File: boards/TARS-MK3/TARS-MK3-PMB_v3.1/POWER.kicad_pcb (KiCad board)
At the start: 2 copper layers, 86 x 79.1 mm, 57 parts, among them J1 Conn_02x12_Odd_Even, J2 Conn_02x12_Odd_Even, J3 Conn_02x12_Odd_Even, J4 Conn_02x12_Odd_Even, J5 AVRISP, U1 LK112M33TR, U2 ATmega328P-A, U3 D36V50F6, U4 D36V50F6, U5 D36V28F9, U6 D36V28F3, U7 D24V50F5, Y1 8Mhz

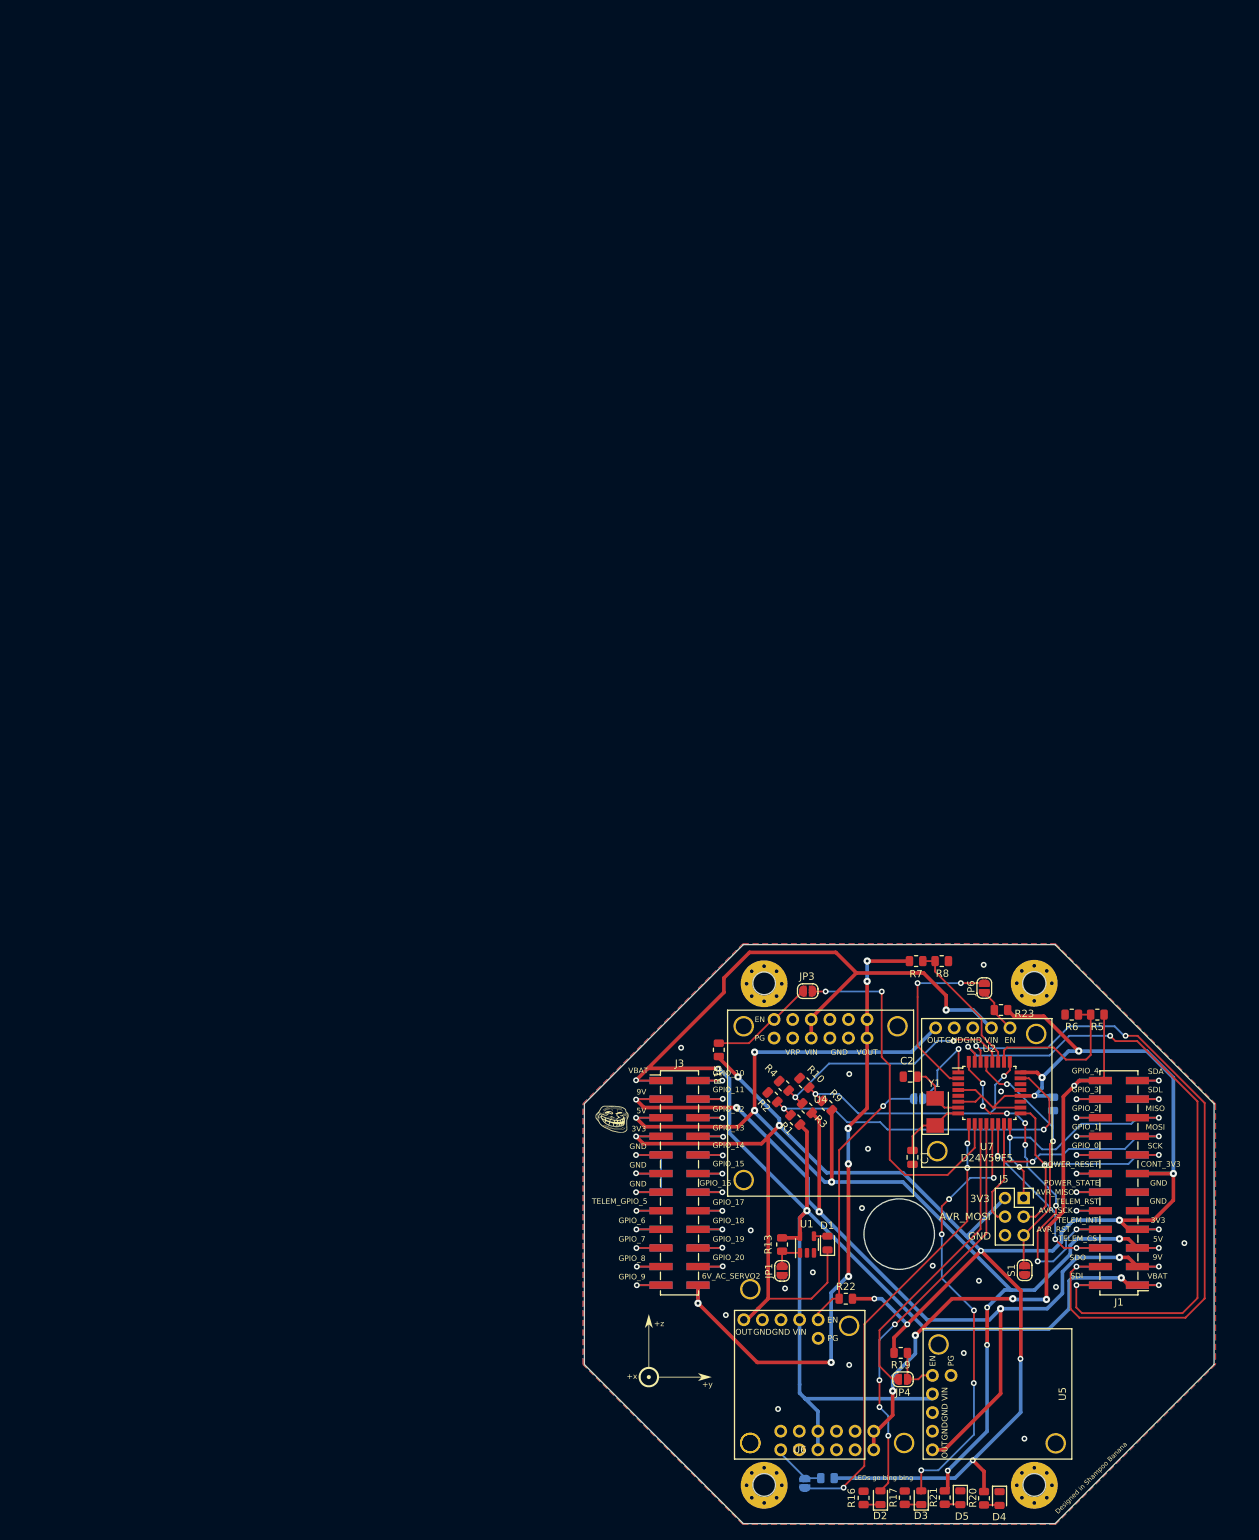
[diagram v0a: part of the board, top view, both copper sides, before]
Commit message: finished template stuff
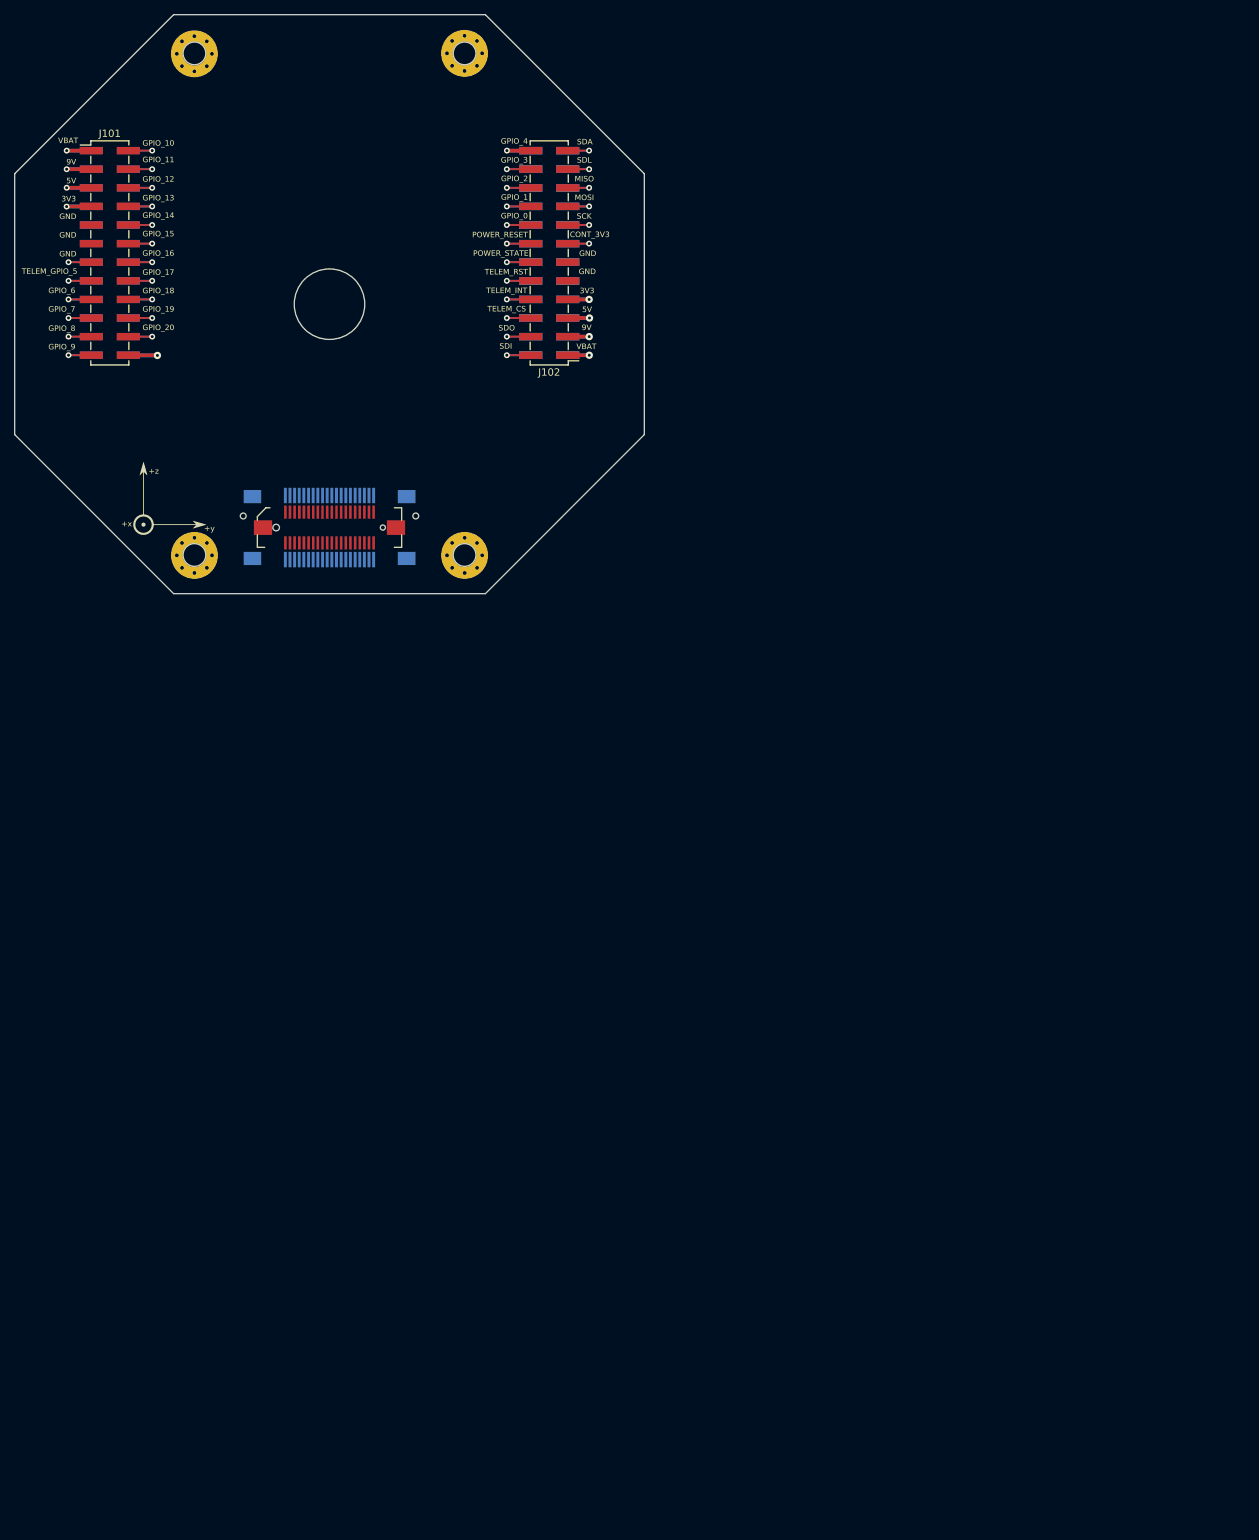
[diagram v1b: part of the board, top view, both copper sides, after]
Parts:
- removed C1, C2: LOAD_C, Capacitor_SMD:C_0805_2012Metric
- removed D1: D, Diode_SMD:D_0805_2012Metric
- removed D2: GREEN, LED_SMD:LED_0805_2012Metric
- removed D3: ORANGE, LED_SMD:LED_0805_2012Metric
- removed D4: LED, LED_SMD:LED_0805_2012Metric
- removed D5: LED, Diode_SMD:D_0805_2012Metric
- removed the G*** at (38.6, 111.3)
- removed the G*** at (101.9, 95.2)
- removed the G*** at (105.1, 141.3)
- removed the G*** at (95.1, 152.1)
- removed J1, J2, J3, J4: Conn_02x12_Odd_Even, Connector_PinHeader_2.54mm:PinHeader_2x12_P2.54mm_Vertical_SMD
- removed J5: AVRISP, Connector_PinSocket_2.54mm:PinSocket_2x03_P2.54mm_Vertical
- removed JP1, JP2, JP3, JP4, JP5, JP6: Jumper_2_Open, Jumper:SolderJumper-2_P1.3mm_Open_RoundedPad1.0x1.5mm
- removed R1, R3: 200kOhm, Resistor_SMD:R_0805_2012Metric
- removed R10, R13, R14, R15, R19, R2, R22, R23, R4, R5, R6, R7, R8, R9: 100kOhm, Resistor_SMD:R_0805_2012Metric
- removed R16, R17: 150Ω, Resistor_SMD:R_0805_2012Metric
- removed R18: 10k, Resistor_SMD:R_0805_2012Metric
- removed R20, R21: 1k, Resistor_SMD:R_0805_2012Metric
- removed the REF** at (96.2, 92.7)
- removed the REF** at (59.3, 92.8)
- removed the REF** at (59.4, 161.3)
- removed the REF** at (96.2, 161.3)
- removed S1: Reset, Jumper:SolderJumper-2_P1.3mm_Open_RoundedPad1.0x1.5mm
- removed U1: LK112M33TR, Package_TO_SOT_SMD:SOT-23-5
- removed U2: ATmega328P-A, Package_QFP:TQFP-32_7x7mm_P0.8mm
- removed U3, U4: D36V50F6, D36V50F6:D36V50F6-TARS
- removed U5: D36V28F9, D36V28F3:D36V28F3
- removed U6: D36V28F3, D36V28F3:D36V28F3
- removed U7: D24V50F5, D24V50F5:D24V50F5
- removed Y1: 8Mhz, Crystal:Crystal_SMD_5032-2Pin_5.0x3.2mm
- added J101: Conn_02x12_Odd_Even, Connector_PinHeader_2.54mm:PinHeader_2x12_P2.54mm_Vertical_SMD, F.Cu at (-30.0, -7.00)
- added J102: Conn_02x12_Odd_Even, Connector_PinHeader_2.54mm:PinHeader_2x12_P2.54mm_Vertical_SMD, F.Cu at (30.0, -7.00)
- added J102, J104: Conn_02x12_Odd_Even, Connector_PinHeader_2.54mm:PinHeader_2x12_P2.54mm_Vertical_SMD, B.Cu at (30.0, -7.00)
- added J103: Conn_02x12_Odd_Even, Connector_PinHeader_2.54mm:PinHeader_2x12_P2.54mm_Vertical_SMD, B.Cu at (-30.0, -7.00)
- added J105: Receptacle, Connector_ISS:2091680401, B.Cu at (0.00, 30.5)
- added J106: 536270474, Connector_ISS:536270474, F.Cu at (0.00, 30.5)
- added REF**: MountingHole_3.2mm_M3_Pad_Via, MountingHole:MountingHole_3.2mm_M3_Pad_Via, F.Cu at (-18.4, 34.3)
- added REF**: MountingHole_3.2mm_M3_Pad_Via, MountingHole:MountingHole_3.2mm_M3_Pad_Via, F.Cu at (18.4, -34.2)
- added REF**: MountingHole_3.2mm_M3_Pad_Via, MountingHole:MountingHole_3.2mm_M3_Pad_Via, F.Cu at (18.4, 34.3)
- added REF**: MountingHole_3.2mm_M3_Pad_Via, MountingHole:MountingHole_3.2mm_M3_Pad_Via, F.Cu at (-18.4, -34.2)
- moved G*** 135.3 mm to (-21.8, 26.5)
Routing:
- net 3V3: track 337.1 -> 0.00 mm, vias 14 -> 0
- net VBAT: track 248.3 -> 0.00 mm, vias 6 -> 0
- net 5V: track 173.1 -> 0.00 mm, vias 9 -> 0
- net 9V: track 139.6 -> 0.00 mm, vias 6 -> 0
- net /B2B_UART_SDO: track 98.5 -> 6.53 mm, vias 3 -> 1
- net /B2B_UART_SDI: track 93.3 -> 6.53 mm, vias 3 -> 1
- net 6V_AC_SERVO2: track 89.2 -> 7.97 mm, vias 7 -> 1
- net 6V_AC_SERVO1: track 85.8 -> 6.51 mm, vias 5 -> 1
- net /6V_AC_SERVO1_EN: track 62.1 -> 0.00 mm, vias 3 -> 0
- net /LED1: track 61.6 -> 0.00 mm, vias 6 -> 0
- net /LED0: track 57.4 -> 0.00 mm, vias 4 -> 0
- net /6V_AC_SERVO2_EN: track 50.1 -> 0.00 mm, vias 2 -> 0
- net /VBAT_MONITOR: track 48.8 -> 0.00 mm, vias 2 -> 0
- net /TELEM_INT: track 49.6 -> 6.53 mm, vias 8 -> 1
- net /9V_EN: track 42.1 -> 0.00 mm
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- removed copper zone on B.Cu, net GND
- removed copper zone on F.Cu, net GND
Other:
- outline, holes or cut-outs redrawn
- board text removed: "6V_AC_SERVO2"
- board text removed: "AVR_MISO"
- board text removed: "AVR_MOSI"
- board text removed: "AVR_RST"
- board text removed: "AVR_SCK"
- board text removed: "Buffett, Arna, Daniel, Rohini, Eisha, Jason, Sam, Rishi, Brian, Alex, Gautam, Ary"
- board text removed: "Designed in Shampoo Banana"
- board text removed: "ILLINOIS SPACE SOCIETY"
- board text removed: "LEDs go bing bing"
- board text removed: "TARS-MK3 Power Management Board Rev.A"
